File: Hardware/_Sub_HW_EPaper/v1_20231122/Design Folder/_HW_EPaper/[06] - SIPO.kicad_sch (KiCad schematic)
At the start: 3 parts, among them U601 74VHC164FT

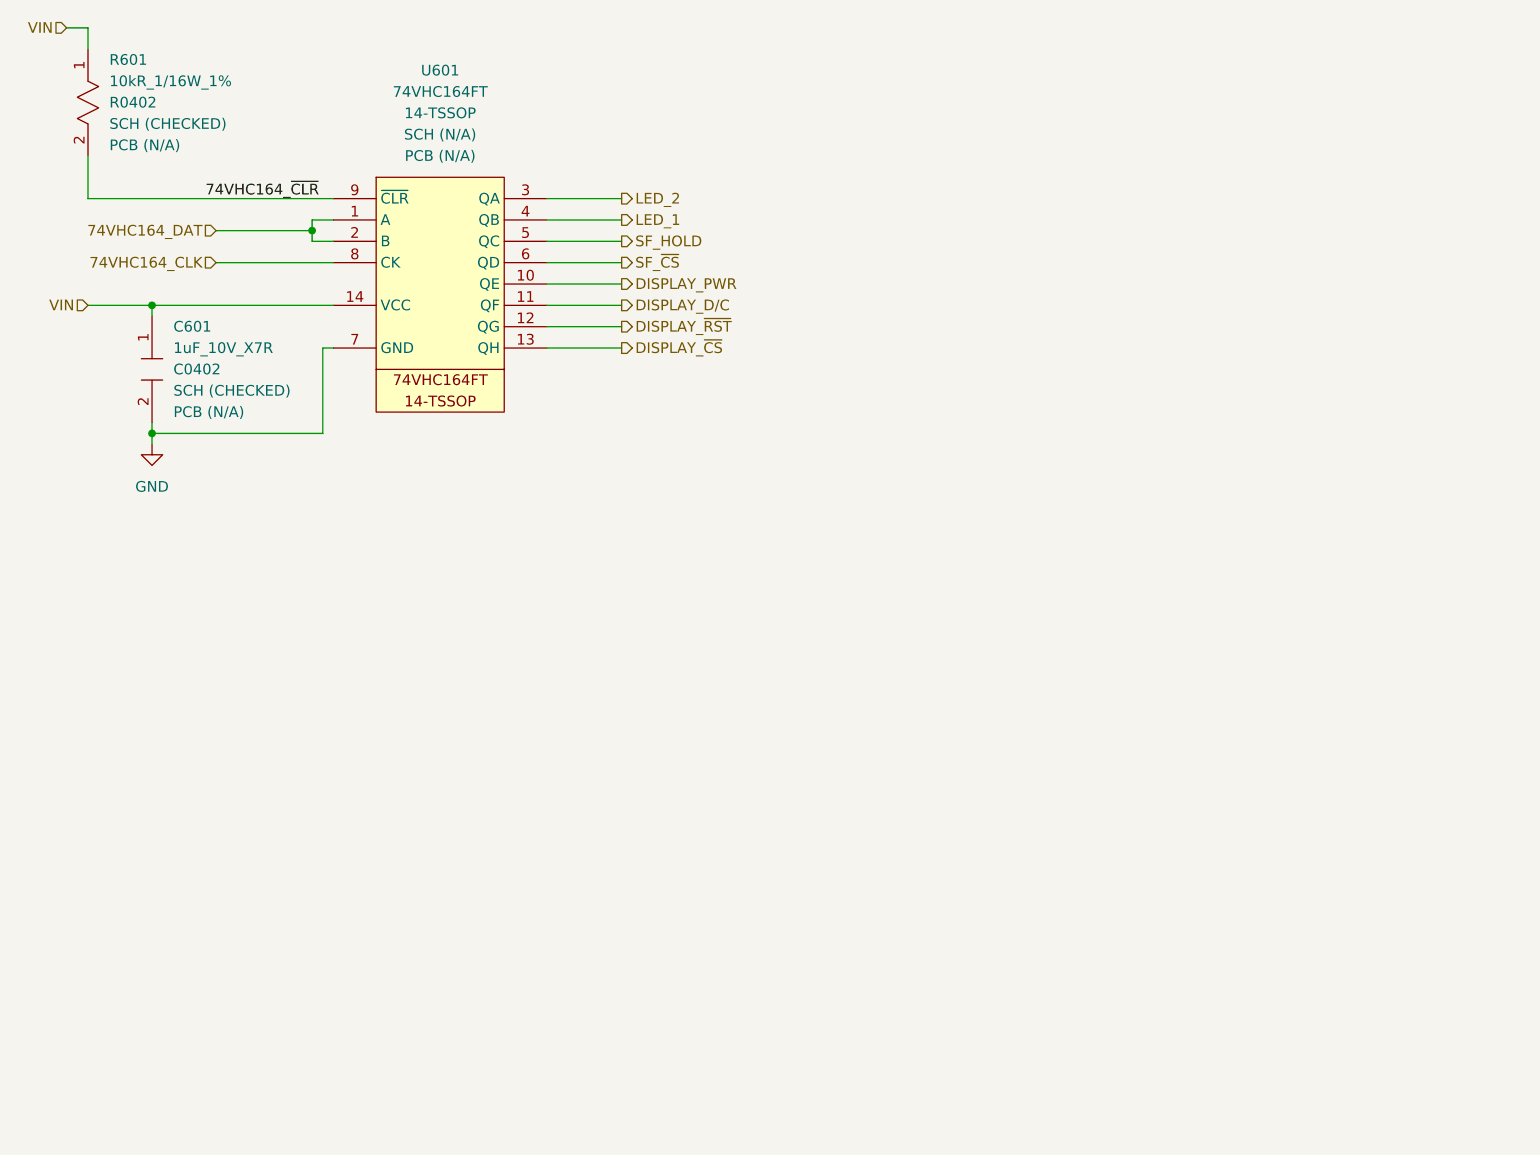
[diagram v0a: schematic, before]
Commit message: Updating file templates and structures...
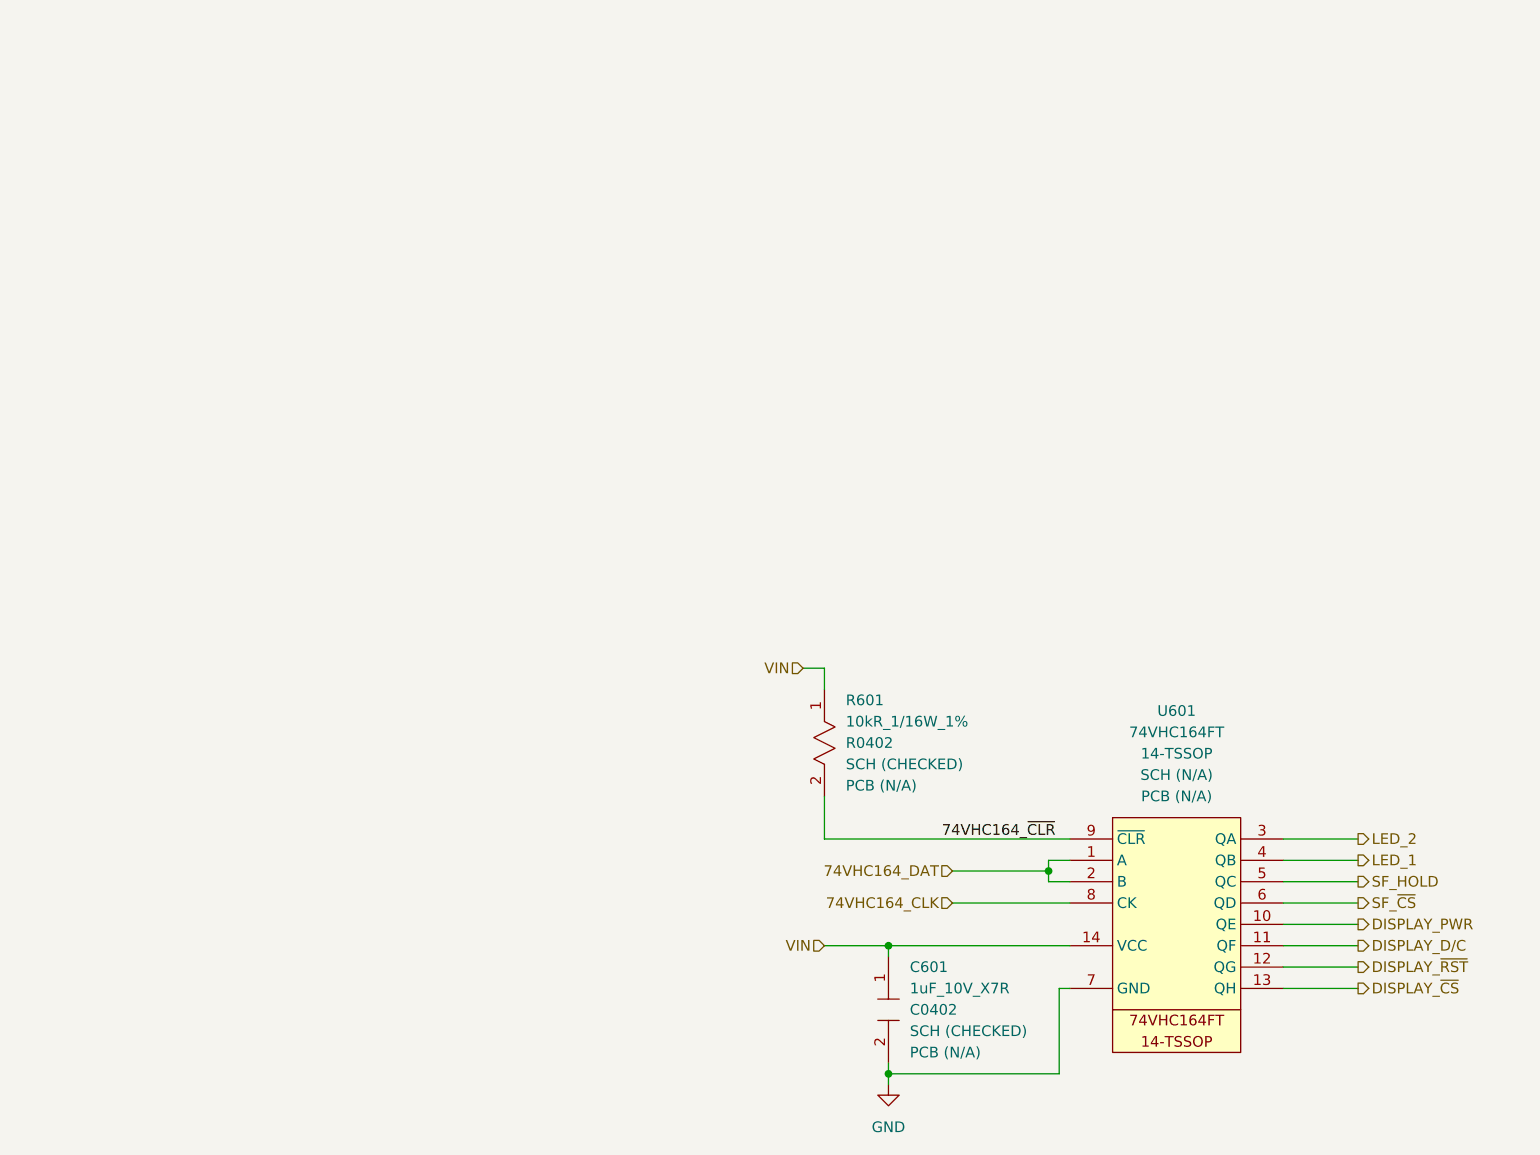
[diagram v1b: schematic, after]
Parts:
- C601: Manufacturer (none) -> Murata Electronics; Part Number GRM155Z71A105KE01D -> (none); Part Number (Manufacturer) (none) -> GRM155Z71A105KE01D; Part Number (Vendor) (none) -> 490-GRM155Z71A105KE01DTR-ND; Vendor (none) -> Digikey
- R601: Manufacturer (none) -> Bourns Inc.; Part Number CR0402-FX-1002GLF -> (none); Part Number (Manufacturer) (none) -> CR0402-FX-1002GLF; Part Number (Vendor) (none) -> CR0402-FX-1002GLFTR-ND; Vendor (none) -> Digikey
- U601: Manufacturer (none) -> Toshiba Semiconductor and Storage; Part Number 74VHC164FT -> (none); Part Number (Manufacturer) (none) -> 74VHC164FT; Part Number (Vendor) (none) -> 264-74VHC164FTTR-ND; Vendor (none) -> Digikey
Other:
- moved on the sheet: C601, R601, U601
